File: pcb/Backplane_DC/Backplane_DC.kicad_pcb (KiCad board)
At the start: 2 copper layers, 100 x 100 mm, 4 parts, among them J1 413638-E, J2 413638-E

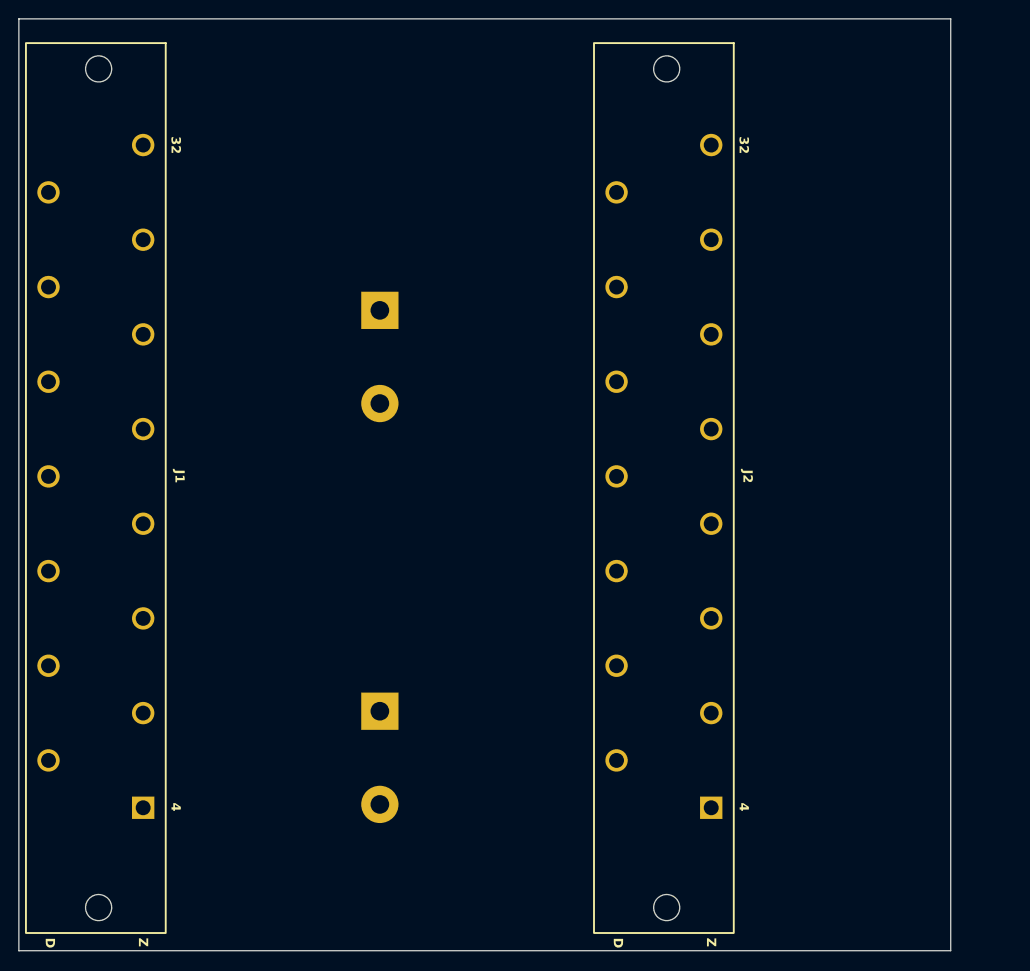
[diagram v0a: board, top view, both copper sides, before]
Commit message: backplane + external lib
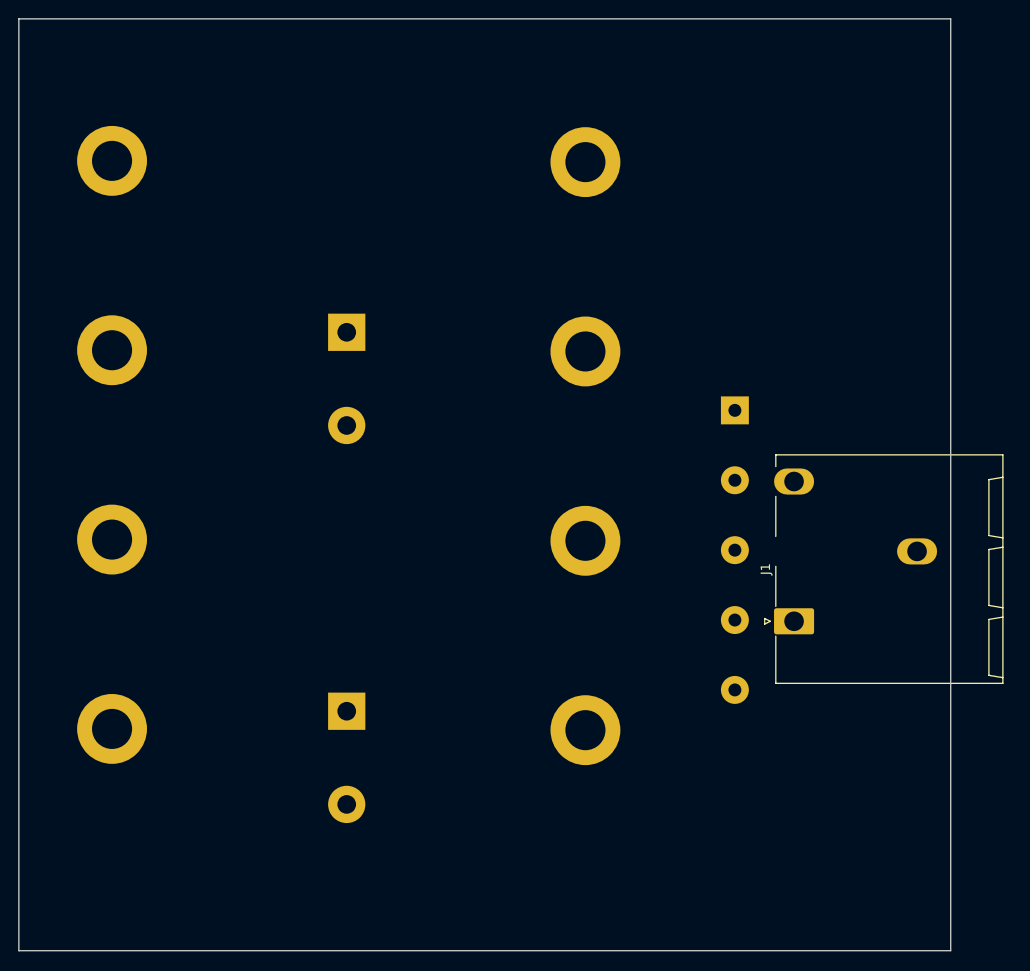
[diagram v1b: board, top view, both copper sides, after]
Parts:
- removed J2: 413638-E, My_Connector:TE_594750-E
- added D1: DNA40U2200GU, Diode_THT:Diode_Bridge_IXYS_GUFP, B.Cu at (116.8, 82.0)
- added H1: MountingHole_Pad, MountingHole:MountingHole_4.3mm_M4_DIN965_Pad, B.Cu at (100.8, 55.4)
- added H2: MountingHole_Pad, MountingHole:MountingHole_4.3mm_M4_DIN965_Pad, B.Cu at (50.0, 55.2)
- added H3: MountingHole_Pad, MountingHole:MountingHole_4.3mm_M4_DIN965_Pad, B.Cu at (50.0, 75.6)
- added H4: MountingHole_Pad, MountingHole:MountingHole_4.3mm_M4_DIN965_Pad, B.Cu at (100.8, 75.7)
- added H5: MountingHole_Pad, MountingHole:MountingHole_4.3mm_M4_DIN965_Pad, B.Cu at (50.0, 95.9)
- added H6: MountingHole_Pad, MountingHole:MountingHole_4.3mm_M4_DIN965_Pad, B.Cu at (100.8, 96.0)
- added H7: MountingHole_Pad, MountingHole:MountingHole_4.3mm_M4_DIN965_Pad, B.Cu at (50.0, 116.2)
- added H8: MountingHole_Pad, MountingHole:MountingHole_4.3mm_M4_DIN965_Pad, B.Cu at (100.8, 116.3)
- J1: value 413638-E -> Conn_01x03; footprint My_Connector:TE_594750-E -> Connector_Phoenix_SPT:PhoenixContact_SPT_5_3-H-7.5-ZB_1x03_P7.5mm_Horizontal
- moved J1 76.5 mm to (123.2, 104.6), turned to 90 degrees
- moved C1 4.27 mm to (75.2, 73.6)
- moved C2 3.56 mm to (75.2, 114.3)
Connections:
- C1 pad 1: unconnected-(C1-Pad1) -> /dcp
- C1 pad 2: unconnected-(C1-Pad2) -> /dcm
- C2 pad 1: unconnected-(C2-Pad1) -> /dcm
- C2 pad 2: unconnected-(C2-Pad2) -> /dcn

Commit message: backplane
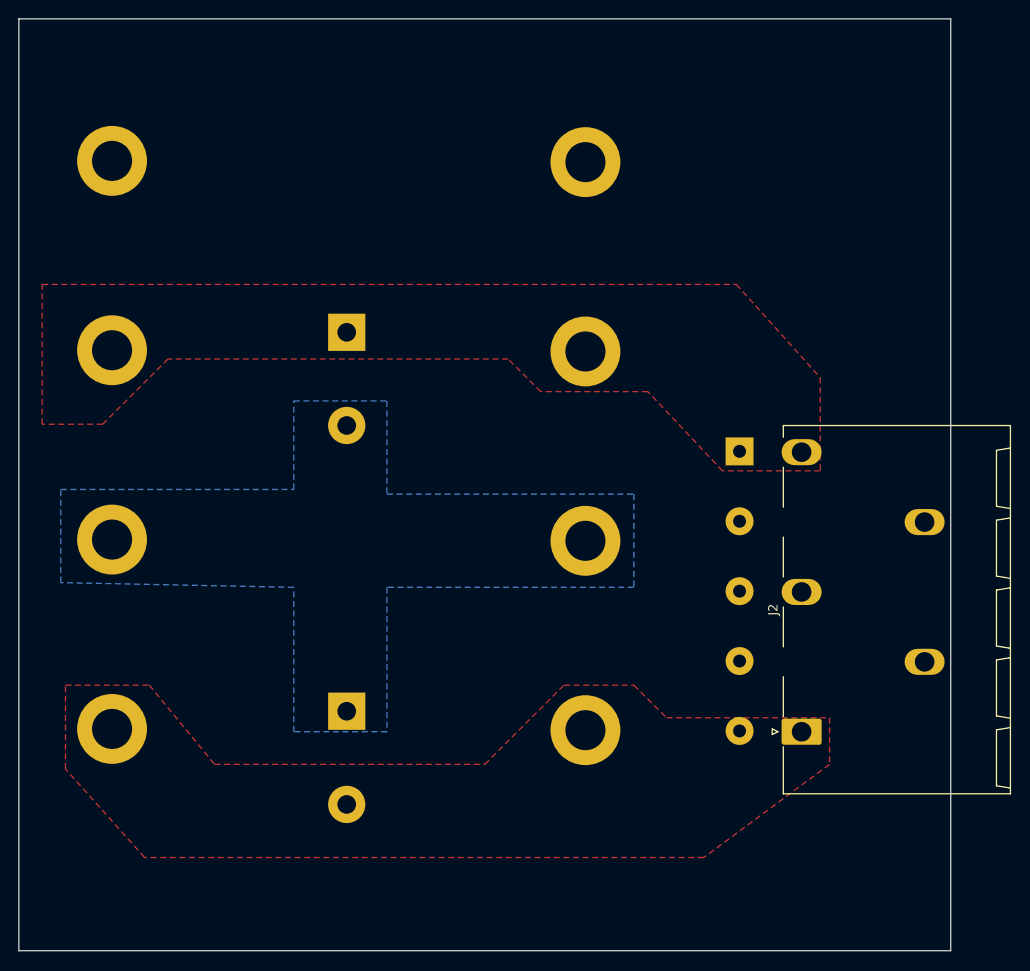
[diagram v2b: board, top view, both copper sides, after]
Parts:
- removed J1: Conn_01x03, Connector_Phoenix_SPT:PhoenixContact_SPT_5_3-H-7.5-ZB_1x03_P7.5mm_Horizontal
- added J2: Conn_01x05, Connector_Phoenix_SPT:PhoenixContact_SPT_5_5-H-7.5-ZB_1x05_P7.5mm_Horizontal, F.Cu at (124.0, 116.5)
- moved D1 4.43 mm to (117.3, 86.4)
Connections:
- D1 pad 2: unconnected-(D1-Pad2) -> /l1
- D1 pad 3: unconnected-(D1-Pad3) -> /l2
- D1 pad 4: unconnected-(D1-Pad4) -> /l3
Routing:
- added copper zone on B.Cu, net /dcm
- added copper zone on F.Cu, net /dcn
- added copper zone on F.Cu, net /dcp
